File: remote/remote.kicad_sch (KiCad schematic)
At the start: 11 parts, among them J4 Screw_Terminal_01x05

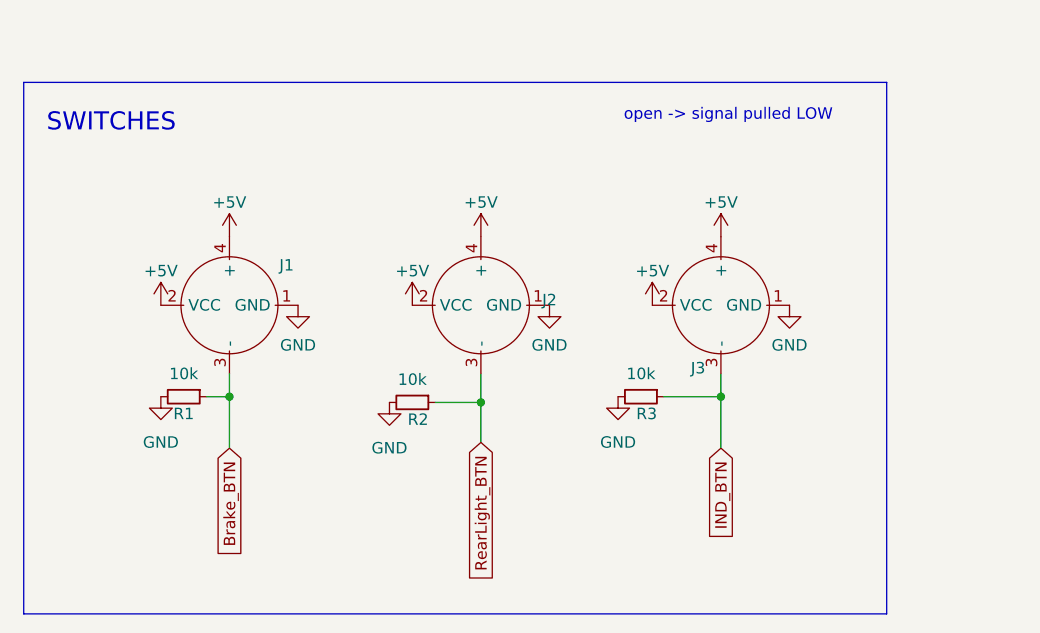
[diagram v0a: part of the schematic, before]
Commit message: generated new fabrication files
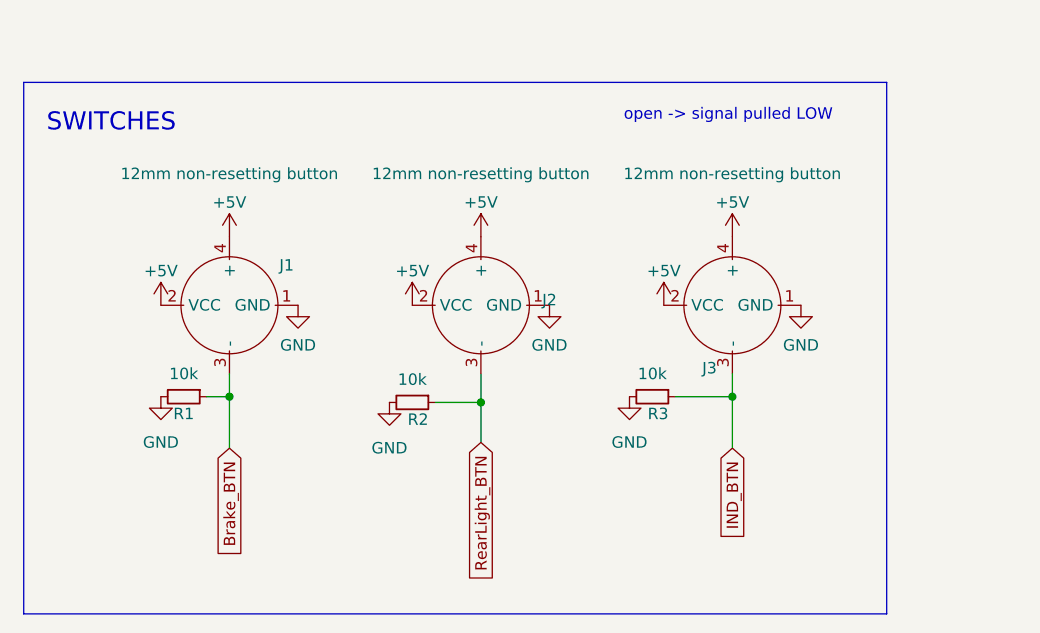
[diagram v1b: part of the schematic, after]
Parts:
- J1, J2, J3: value ~ -> 12mm non-resetting button
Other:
- moved on the sheet: J3, R3
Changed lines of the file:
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@@
   (junction (at 236.22 32.385) (diameter 0) (color 0 0 0 0)
   )
-  (junction (at 92.71 89.535) (diameter 0) (color 0 0 0 0)
+  (junction (at 93.98 89.535) (diameter 0) (color 0 0 0 0)
   )
   (junction (at 187.96 32.385) (diameter 0) (color 0 0 0 0)
@@
   (junction (at 50.165 24.13) (diameter 0) (color 0 0 0 0)
   )
-  (wire (pts (xy 92.71 89.535) (xy 92.71 86.995))
+  (wire (pts (xy 93.98 89.535) (xy 93.98 86.995))
     (stroke (width 0) (type default))
   )
@@
     (stroke (width 0) (type default))
   )
-  (wire (pts (xy 92.71 95.25) (xy 92.71 89.535))
+  (wire (pts (xy 93.98 95.25) (xy 93.98 89.535))
     (stroke (width 0) (type default))
   )
@@
     (stroke (width 0) (type default))
   )
-  (wire (pts (xy 92.71 89.535) (xy 86.36 89.535))
+  (wire (pts (xy 93.98 89.535) (xy 87.63 89.535))
     (stroke (width 0) (type default))
   )
@@
     )
   )
-  (global_label "IND_BTN" (shape input) (at 92.71 95.25 270) (fields_autoplaced)
+  (global_label "IND_BTN" (shape input) (at 93.98 95.25 270) (fields_autoplaced)
     (effects (font (size 1.27 1.27)) (justify right))
-    (property "Intersheetrefs" "${INTERSHEET_REFS}" (at 92.71 105.8968 90)
+    (property "Intersheetrefs" "${INTERSHEET_REFS}" (at 93.98 105.8968 90)
       (effects (font (size 1.27 1.27)) (justify right) hide)
     )
@@
       (effects (font (size 1.27 1.27)))
     )
-    (property "Value" "~" (at 38.1 79.375 0)
+    (property "Value" "12mm non-resetting button" (at 38.1 64.77 0)
       (effects (font (size 1.27 1.27)))
     )
@@
   )
   (symbol (lib_id "Button_Switch:5V_LED_SWITCH") (at 66.04 79.375 0) (unit 1)
-    (in_bom yes) (on_board yes) (dnp no) (fields_autoplaced)
+    (in_bom yes) (on_board yes) (dnp no)
     (property "Reference" "J2" (at 73.66 78.7909 0)
       (effects (font (size 1.27 1.27)))
     )
-    (property "Value" "~" (at 66.04 79.375 0)
+    (property "Value" "12mm non-resetting button" (at 66.04 64.77 0)
       (effects (font (size 1.27 1.27)))
     )
@@
     )
   )
-  (symbol (lib_id "power:GND") (at 100.33 79.375 0) (unit 1)
-    (in_bom yes) (on_board yes) (dnp no) (fields_autoplaced)
-    (property "Reference" "#PWR09" (at 100.33 85.725 0)
-      (effects (font (size 1.27 1.27)) hide)
-    )
-    (property "Value" "GND" (at 100.33 83.82 0)
-      (effects (font (size 1.27 1.27)))
-    )
-    (property "Footprint" "" (at 100.33 79.375 0)
-      (effects (font (size 1.27 1.27)) hide)
-    )
-    (property "Datasheet" "" (at 100.33 79.375 0)
+  (symbol (lib_id "power:GND") (at 101.6 79.375 0) (unit 1)
+    (in_bom yes) (on_board yes) (dnp no) (fields_autoplaced)
+    (property "Reference" "#PWR09" (at 101.6 85.725 0)
+      (effects (font (size 1.27 1.27)) hide)
+    )
+    (property "Value" "GND" (at 101.6 83.82 0)
+      (effects (font (size 1.27 1.27)))
+    )
+    (property "Footprint" "" (at 101.6 79.375 0)
+      (effects (font (size 1.27 1.27)) hide)
+    )
+    (property "Datasheet" "" (at 101.6 79.375 0)
       (effects (font (size 1.27 1.27)) hide)
     )
@@
     )
   )
-  (symbol (lib_id "power:+5V") (at 85.09 79.375 0) (unit 1)
-    (in_bom yes) (on_board yes) (dnp no) (fields_autoplaced)
-    (property "Reference" "#PWR05" (at 85.09 83.185 0)
-      (effects (font (size 1.27 1.27)) hide)
-    )
-    (property "Value" "+5V" (at 85.09 75.565 0)
-      (effects (font (size 1.27 1.27)))
-    )
-    (property "Footprint" "" (at 85.09 79.375 0)
-      (effects (font (size 1.27 1.27)) hide)
-    )
-    (property "Datasheet" "" (at 85.09 79.375 0)
+  (symbol (lib_id "power:+5V") (at 86.36 79.375 0) (unit 1)
+    (in_bom yes) (on_board yes) (dnp no) (fields_autoplaced)
+    (property "Reference" "#PWR05" (at 86.36 83.185 0)
+      (effects (font (size 1.27 1.27)) hide)
+    )
+    (property "Value" "+5V" (at 86.36 75.565 0)
+      (effects (font (size 1.27 1.27)))
+    )
+    (property "Footprint" "" (at 86.36 79.375 0)
+      (effects (font (size 1.27 1.27)) hide)
+    )
+    (property "Datasheet" "" (at 86.36 79.375 0)
       (effects (font (size 1.27 1.27)) hide)
     )
@@
     )
   )
-  (symbol (lib_id "Device:R_Small") (at 83.82 89.535 270) (unit 1)
+  (symbol (lib_id "Device:R_Small") (at 85.09 89.535 270) (unit 1)
     (in_bom yes) (on_board yes) (dnp no)
-    (property "Reference" "R3" (at 84.455 91.44 90)
-      (effects (font (size 1.27 1.27)))
-    )
-    (property "Value" "10k" (at 83.82 86.995 90)
-      (effects (font (size 1.27 1.27)))
-    )
-    (property "Footprint" "Resistor_SMD:R_0603_1608Metric" (at 83.82 89.535 0)
-      (effects (font (size 1.27 1.27)) hide)
-    )
-    (property "Datasheet" "~" (at 83.82 89.535 0)
+    (property "Reference" "R3" (at 85.725 91.44 90)
+      (effects (font (size 1.27 1.27)))
+    )
+    (property "Value" "10k" (at 85.09 86.995 90)
+      (effects (font (size 1.27 1.27)))
+    )
+    (property "Footprint" "Resistor_SMD:R_0603_1608Metric" (at 85.09 89.535 0)
+      (effects (font (size 1.27 1.27)) hide)
+    )
+    (property "Datasheet" "~" (at 85.09 89.535 0)
       (effects (font (size 1.27 1.27)) hide)
     )
@@
     )
   )
-  (symbol (lib_id "power:GND") (at 81.28 89.535 0) (unit 1)
-    (in_bom yes) (on_board yes) (dnp no) (fields_autoplaced)
-    (property "Reference" "#PWR011" (at 81.28 95.885 0)
-      (effects (font (size 1.27 1.27)) hide)
-    )
-    (property "Value" "GND" (at 81.28 94.615 0)
-      (effects (font (size 1.27 1.27)))
-    )
-    (property "Footprint" "" (at 81.28 89.535 0)
-      (effects (font (size 1.27 1.27)) hide)
-    )
-    (property "Datasheet" "" (at 81.28 89.535 0)
+  (symbol (lib_id "power:GND") (at 82.55 89.535 0) (unit 1)
+    (in_bom yes) (on_board yes) (dnp no) (fields_autoplaced)
+    (property "Reference" "#PWR011" (at 82.55 95.885 0)
+      (effects (font (size 1.27 1.27)) hide)
+    )
+    (property "Value" "GND" (at 82.55 94.615 0)
+      (effects (font (size 1.27 1.27)))
+    )
+    (property "Footprint" "" (at 82.55 89.535 0)
+      (effects (font (size 1.27 1.27)) hide)
+    )
+    (property "Datasheet" "" (at 82.55 89.535 0)
       (effects (font (size 1.27 1.27)) hide)
     )
@@
     )
   )
-  (symbol (lib_id "Button_Switch:5V_LED_SWITCH") (at 92.71 79.375 0) (unit 1)
+  (symbol (lib_id "Button_Switch:5V_LED_SWITCH") (at 93.98 79.375 0) (unit 1)
     (in_bom yes) (on_board yes) (dnp no)
-    (property "Reference" "J3" (at 90.17 86.36 0)
-      (effects (font (size 1.27 1.27)))
-    )
-    (property "Value" "~" (at 92.71 79.375 0)
-      (effects (font (size 1.27 1.27)))
-    )
-    (property "Footprint" "Button_Switch:5V_LED_BTN" (at 92.71 79.375 0)
-      (effects (font (size 1.27 1.27)) hide)
-    )
-    (property "Datasheet" "" (at 92.71 79.375 0)
+    (property "Reference" "J3" (at 91.44 86.36 0)
+      (effects (font (size 1.27 1.27)))
+    )
+    (property "Value" "12mm non-resetting button" (at 93.98 64.77 0)
+      (effects (font (size 1.27 1.27)))
+    )
+    (property "Footprint" "Button_Switch:5V_LED_BTN" (at 93.98 79.375 0)
+      (effects (font (size 1.27 1.27)) hide)
+    )
+    (property "Datasheet" "" (at 93.98 79.375 0)
       (effects (font (size 1.27 1.27)) hide)
     )
@@
     )
   )
-  (symbol (lib_id "power:+5V") (at 92.71 71.755 0) (unit 1)
-    (in_bom yes) (on_board yes) (dnp no) (fields_autoplaced)
-    (property "Reference" "#PWR014" (at 92.71 75.565 0)
-      (effects (font (size 1.27 1.27)) hide)
-    )
-    (property "Value" "+5V" (at 92.71 67.945 0)
-      (effects (font (size 1.27 1.27)))
-    )
-    (property "Footprint" "" (at 92.71 71.755 0)
-      (effects (font (size 1.27 1.27)) hide)
-    )
-    (property "Datasheet" "" (at 92.71 71.755 0)
-      (effects (font (size 1.27 1.27)) hide)
-    )
+  (symbol (lib_id "power:+5V") (at 93.98 71.755 0) (unit 1)
+    (in_bom yes) (on_board yes) (dnp no) (fields_autoplaced)
+    (property "Reference" "#PWR014" (at 93.98 75.565 0)
+      (effects (font (size 1.27 1.27)) hide)
+    )
+    (property "Value" "+5V" (at 93.98 67.945 0)
+      (effects (font (size 1.27 1.27)))
+    )
+    (property "Footprint" "" (at 93.98 71.755 0)
+      (effects (font (size 1.27 1.27)) hide)
+    )
+    (property "Datasheet" "" (at 93.98 71.755 0)
+      (effects (font (size 1.27 1.27)) hide)
+    )
